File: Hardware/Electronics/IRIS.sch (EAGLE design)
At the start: 24 parts, among them Q2 12MHz, U1 AT32UC3C, U2 TCD1304AP, X2 MINI-USB-32005-201

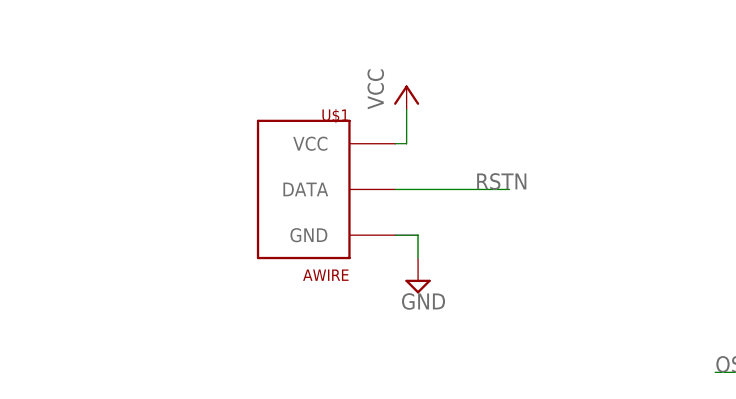
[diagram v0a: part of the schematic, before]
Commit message: First version
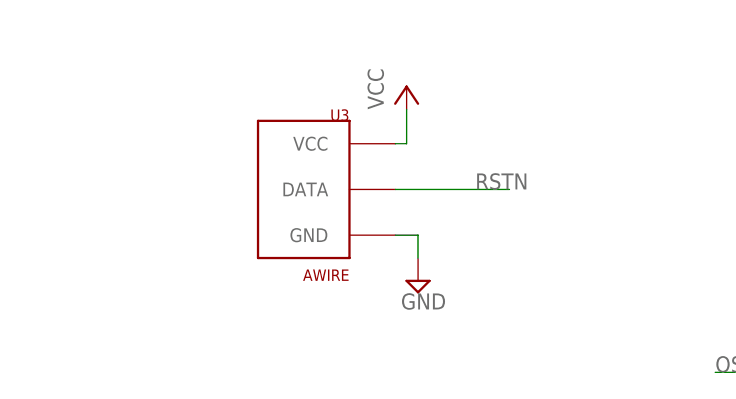
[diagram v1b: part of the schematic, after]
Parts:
- renumbered U$1 to U3
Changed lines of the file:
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@@
 <setting verticaltext="up"/>
 </settings>
-<grid distance="0.05" unitdist="inch" unit="inch" style="lines" multiple="1" display="no" altdistance="0.01" altunitdist="inch" altunit="inch"/>
+<grid distance="0.1" unitdist="inch" unit="inch" style="lines" multiple="1" display="no" altdistance="0.01" altunitdist="inch" altunit="inch"/>
 <layers>
 <layer number="1" name="Top" color="4" fill="1" visible="no" active="no"/>
@@
 <part name="R2" library="rcl" deviceset="R-EU_" device="R0603" value="39"/>
 <part name="C10" library="rcl" deviceset="C-EU" device="C0603" value="100nF"/>
-<part name="U$1" library="IRIS" deviceset="AWIRE" device=""/>
+<part name="U3" library="IRIS" deviceset="AWIRE" device=""/>
 <part name="P+9" library="supply1" deviceset="VCC" device=""/>
 <part name="SUPPLY11" library="supply2" deviceset="GND" device=""/>
@@
 <instance part="R2" gate="G$1" x="130.81" y="6.35"/>
 <instance part="C10" gate="G$1" x="-66.04" y="-33.02"/>
-<instance part="U$1" gate="G$1" x="-46.99" y="95.25" rot="MR0"/>
+<instance part="U3" gate="G$1" x="-46.99" y="95.25" rot="MR0"/>
 <instance part="P+9" gate="VCC" x="-40.64" y="106.68"/>
 <instance part="SUPPLY11" gate="GND" x="-39.37" y="85.09"/>
@@
 </segment>
 <segment>
-<pinref part="U$1" gate="G$1" pin="GND"/>
+<pinref part="U3" gate="G$1" pin="GND"/>
 <wire x1="-41.91" y1="90.17" x2="-39.37" y2="90.17" width="0.1524" layer="91"/>
 <wire x1="-39.37" y1="90.17" x2="-39.37" y2="87.63" width="0.1524" layer="91"/>
@@
 </segment>
 <segment>
-<pinref part="U$1" gate="G$1" pin="VCC"/>
+<pinref part="U3" gate="G$1" pin="VCC"/>
 <wire x1="-41.91" y1="100.33" x2="-40.64" y2="100.33" width="0.1524" layer="91"/>
 <wire x1="-40.64" y1="100.33" x2="-40.64" y2="104.14" width="0.1524" layer="91"/>
@@
 </segment>
 <segment>
-<pinref part="U$1" gate="G$1" pin="DATA"/>
+<pinref part="U3" gate="G$1" pin="DATA"/>
 <wire x1="-41.91" y1="95.25" x2="-29.21" y2="95.25" width="0.1524" layer="91"/>
 <label x="-33.02" y="95.25" size="1.778" layer="95"/>
